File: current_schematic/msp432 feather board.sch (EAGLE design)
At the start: 53 parts, among them IC1 FT232RL, J1 1981568-1, J2 B2B-PH-SM4-TB(LF)(SN), U1 DMG3415U-7X2-DFN2015-3, U2 MCP73831T-2ACI/OT, X1 TSW-116-07-G-S, X2 TSW-116-07-G-S, Y1 ECS-480-10-37-JTN-TR

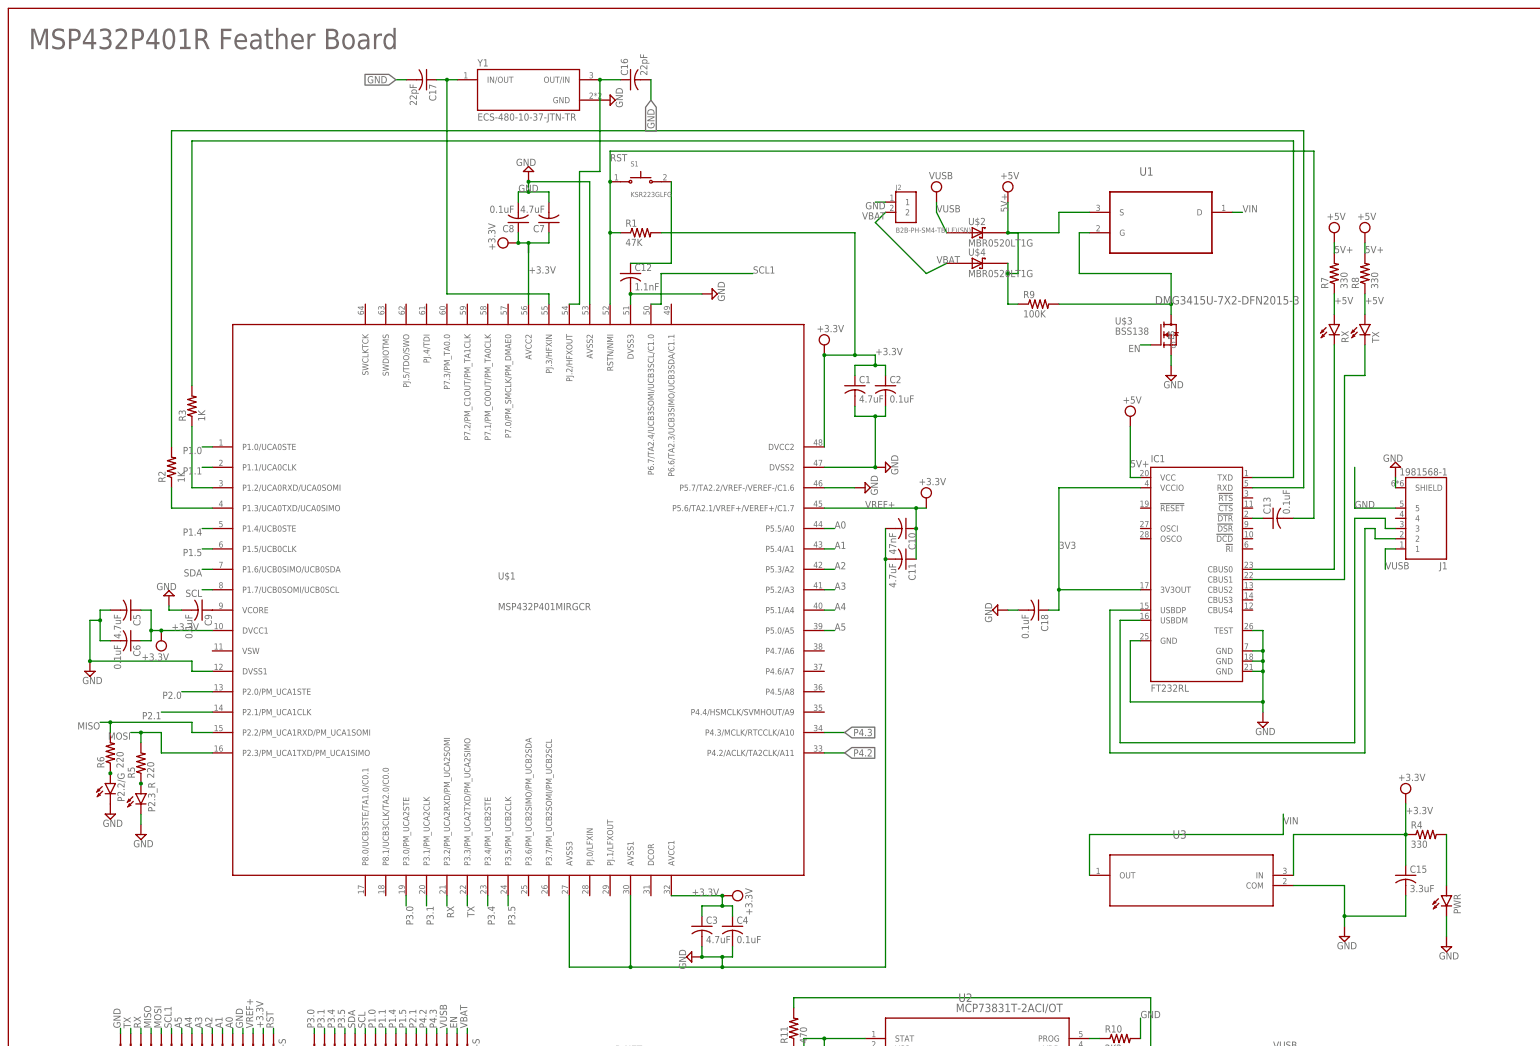
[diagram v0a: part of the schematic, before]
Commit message: Add files via upload
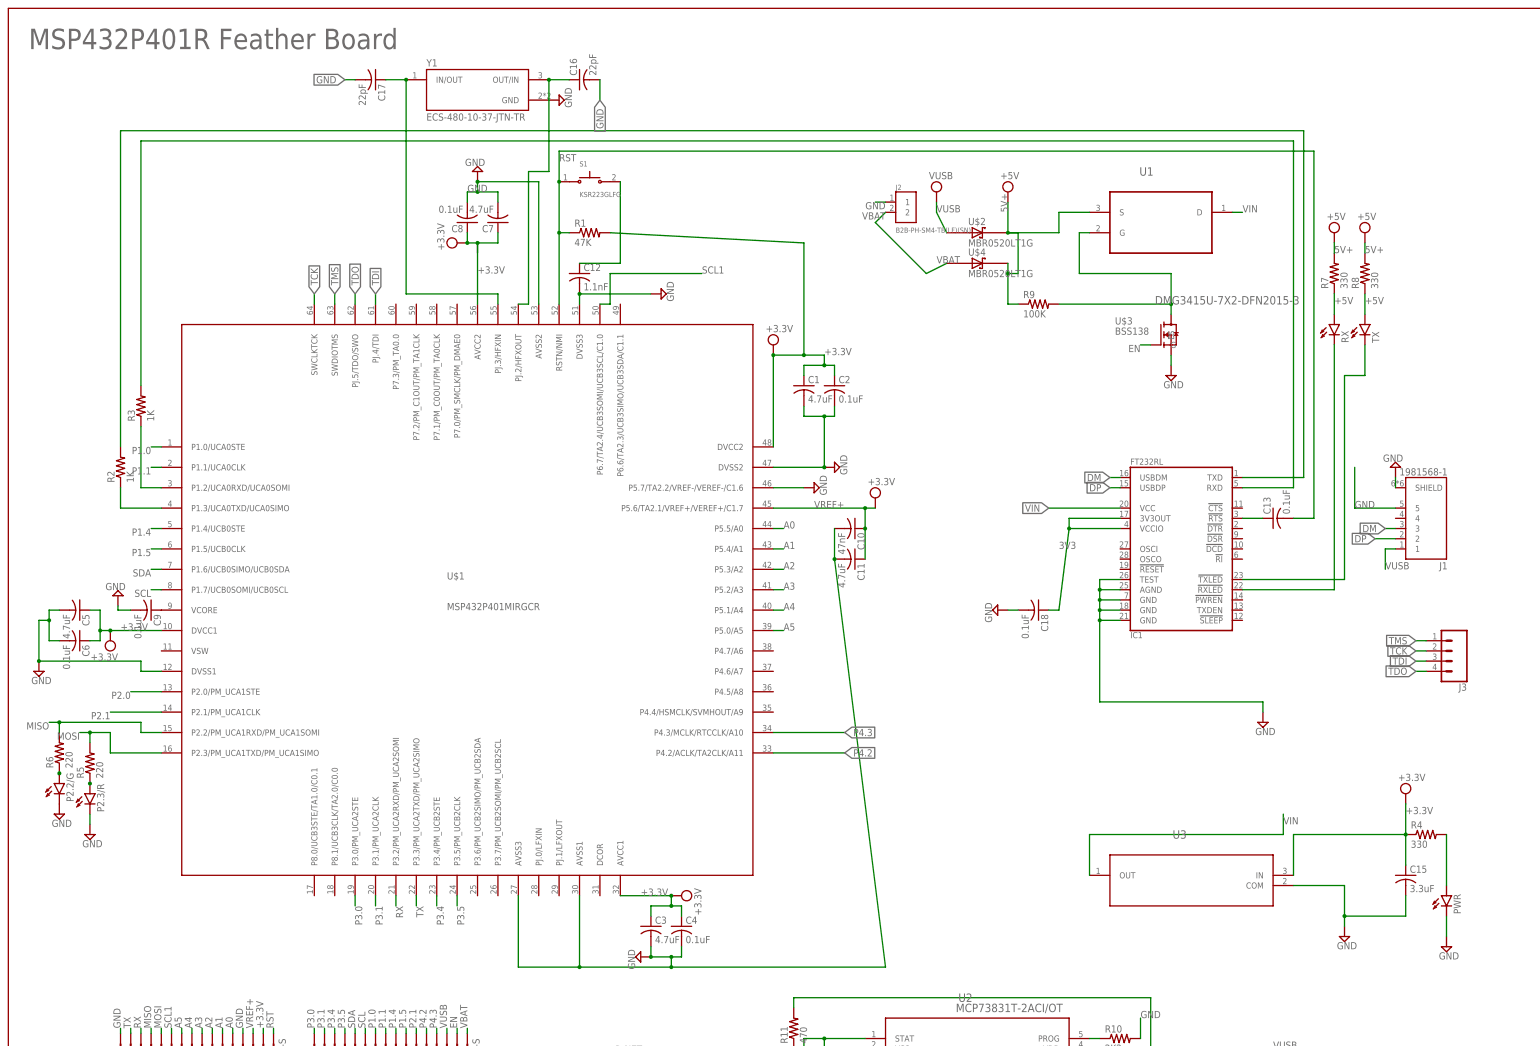
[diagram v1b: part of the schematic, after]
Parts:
- removed P2.3_R: (no value), led:LEDCHIP-LED0603
- added J3: (no value), SparkFun-Connectors:CONN_041X04_NO_SILK
- added P2.3/R: (no value), led:LEDCHIP-LED0603
- IC1: device ftdichip:FT232RL -> FT232RL:FT232RL
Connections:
- net N$5 renamed DM
- net N$6 renamed DP
- new net TCK: J3.2, U$1.SWCLKTCK
- new net TDI: J3.3, U$1.PJ.4/TDI
- new net TDO: J3.4, U$1.PJ.5/TDO/SWO
- new net TMS: J3.1, U$1.SWDIOTMS
- net 5V+: no longer IC1.VCC
- net GND: now also IC1.AGND, IC1.GND@18, IC1.GND@21, IC1.GND@7, P2.3/R.C; no longer IC1.GND, IC1.GND@1, IC1.GND@2, IC1.GND@A, P2.3_R.C
- net N$11: now also IC1.!RXLED; no longer IC1.CBUS0
- net N$12: now also IC1.!TXLED; no longer IC1.CBUS1
- net N$3: now also IC1.!RTS; no longer IC1.!DTR
- net N$42: now also P2.3/R.A; no longer P2.3_R.A
- net N$7: now also IC1.RXD; no longer IC1.TXD
- net N$8: now also IC1.TXD; no longer IC1.RXD
- net VIN: now also IC1.VCC
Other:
- moved on the sheet: C1, C10, C11, C12, C16, C17, C2, C3, C4, C5, C6, C7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
